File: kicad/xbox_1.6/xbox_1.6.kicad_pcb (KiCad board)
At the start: 2 copper layers, 18 parts, among them U2C1 intel_495_bga2, U4B1 ddr_100_tqfp, U4C1 nvidia_xgpu_nv2a, U5F1 ddr_100_tqfp, U6D1 ddr_100_tqfp, U6E1 nvidia_mcpx

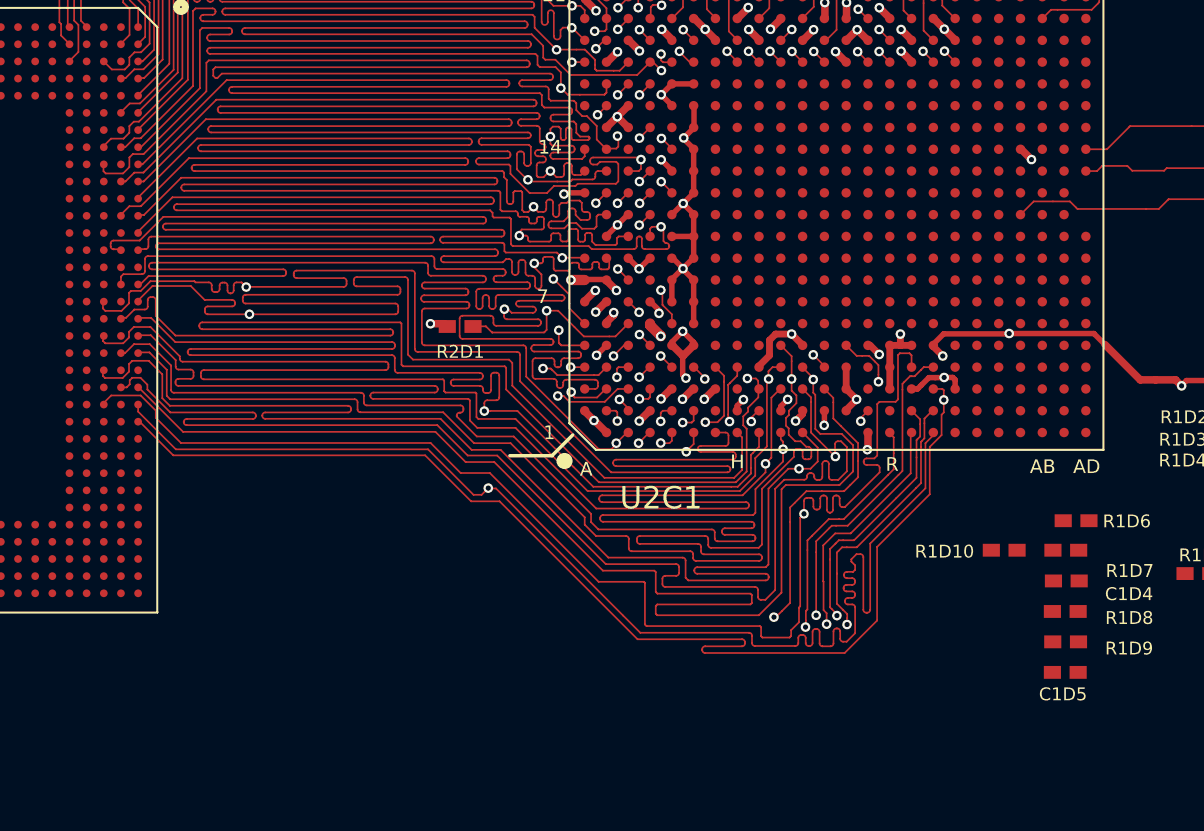
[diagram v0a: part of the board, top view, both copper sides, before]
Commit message: route more
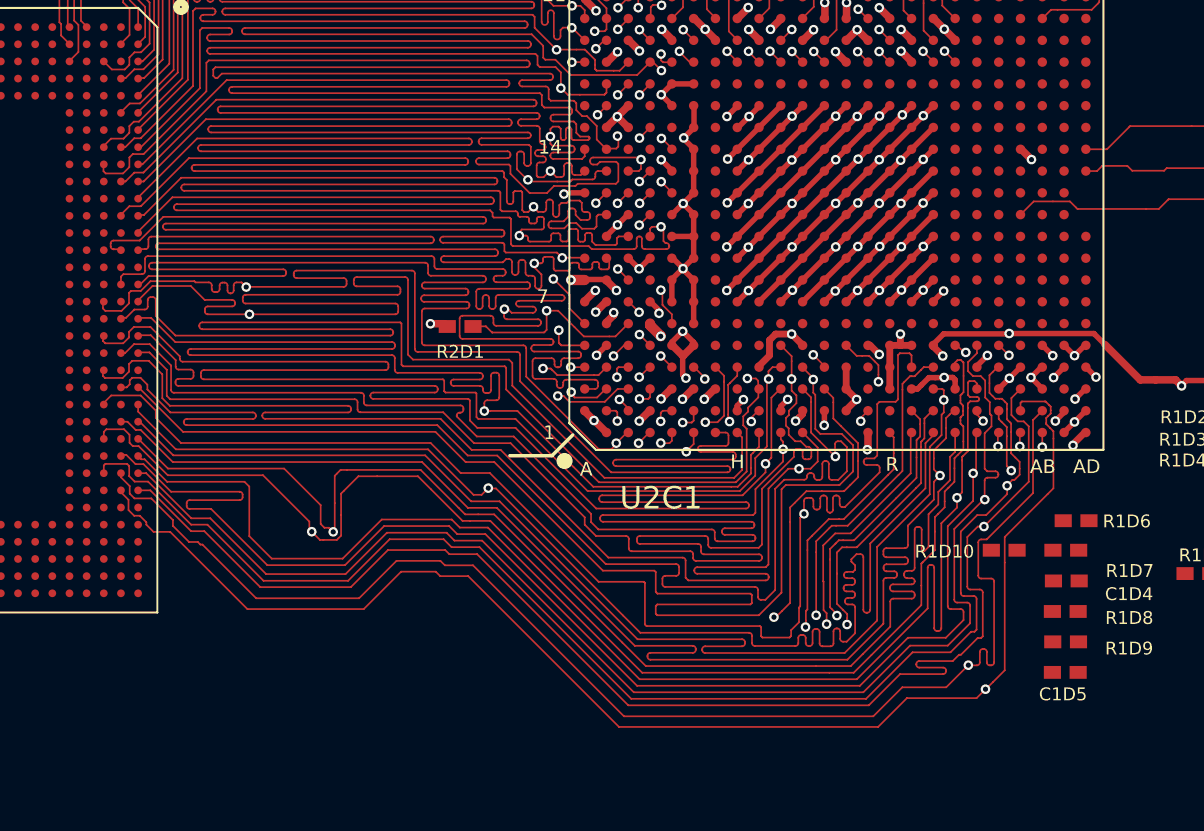
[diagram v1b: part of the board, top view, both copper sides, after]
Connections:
- U2C1 pad AA1: (no net) -> /CPU_AERR
- U2C1 pad AA2: (no net) -> /CPU_RS1
- U2C1 pad AA3: (no net) -> /CPU_DBSY
- U2C1 pad AA4: (no net) -> /VSS
- U2C1 pad AB1: (no net) -> /CPU_AP0
- U2C1 pad AB2: (no net) -> /CPU_ADS
- U2C1 pad AB3: (no net) -> /VSS
- U2C1 pad AB4: (no net) -> /VSS
- U2C1 pad AB5: (no net) -> /VSS
- U2C1 pad AC1: (no net) -> /VSS
- U2C1 pad AC2: (no net) -> /VSS
- U2C1 pad AC4: (no net) -> /VSS
- U2C1 pad AC5: (no net) -> /VSS
- U2C1 pad AD1: (no net) -> /VSS
- U2C1 pad AD2: (no net) -> /VSS
- U2C1 pad AD3: (no net) -> /VSS
- U2C1 pad AD4: (no net) -> /VSS
- U2C1 pad AD5: (no net) -> /VSS
- U2C1 pad H10: (no net) -> /CPU_VCC
- U2C1 pad H11: (no net) -> /VSS
- U2C1 pad H12: (no net) -> /CPU_VCC
- U2C1 pad H13: (no net) -> /VSS
- U2C1 pad H14: (no net) -> /CPU_VCC
- U2C1 pad H15: (no net) -> /VSS
- U2C1 pad H16: (no net) -> /CPU_VCC
- U2C1 pad H7: (no net) -> /VSS
- U2C1 pad H8: (no net) -> /CPU_VCC
- U2C1 pad H9: (no net) -> /VSS
- U2C1 pad J10: (no net) -> /VSS
- U2C1 pad J11: (no net) -> /CPU_VCC
- U2C1 pad J12: (no net) -> /VSS
- U2C1 pad J13: (no net) -> /CPU_VCC
- U2C1 pad J14: (no net) -> /VSS
- U2C1 pad J15: (no net) -> /CPU_VCC
- U2C1 pad J16: (no net) -> /VSS
- U2C1 pad J6: (no net) -> /CPU_VCCT
- U2C1 pad J7: (no net) -> /CPU_VCC
- U2C1 pad J8: (no net) -> /VSS
- U2C1 pad J9: (no net) -> /CPU_VCC
- U2C1 pad K10: (no net) -> /CPU_VCC
- U2C1 pad K11: (no net) -> /VSS
- U2C1 pad K12: (no net) -> /CPU_VCC
- U2C1 pad K13: (no net) -> /VSS
- U2C1 pad K14: (no net) -> /CPU_VCC
- U2C1 pad K15: (no net) -> /VSS
- U2C1 pad K16: (no net) -> /CPU_VCC
- U2C1 pad K7: (no net) -> /VSS
- U2C1 pad K8: (no net) -> /CPU_VCC
- U2C1 pad K9: (no net) -> /VSS
- U2C1 pad L10: (no net) -> /VSS
- U2C1 pad L11: (no net) -> /CPU_VCC
- U2C1 pad L12: (no net) -> /VSS
- U2C1 pad L13: (no net) -> /CPU_VCC
- U2C1 pad L14: (no net) -> /VSS
- U2C1 pad L15: (no net) -> /CPU_VCC
- U2C1 pad L16: (no net) -> /VSS
- U2C1 pad L7: (no net) -> /CPU_VCC
- U2C1 pad L8: (no net) -> /VSS
- U2C1 pad L9: (no net) -> /CPU_VCC
- U2C1 pad M10: (no net) -> /CPU_VCC
- U2C1 pad M11: (no net) -> /VSS
- U2C1 pad M12: (no net) -> /CPU_VCC
- U2C1 pad M13: (no net) -> /VSS
- U2C1 pad M14: (no net) -> /CPU_VCC
- U2C1 pad M15: (no net) -> /VSS
- U2C1 pad M16: (no net) -> /CPU_VCC
- U2C1 pad M7: (no net) -> /VSS
- U2C1 pad M8: (no net) -> /CPU_VCC
- U2C1 pad M9: (no net) -> /VSS
- U2C1 pad N10: (no net) -> /VSS
- U2C1 pad N11: (no net) -> /CPU_VCC
- U2C1 pad N12: (no net) -> /VSS
- U2C1 pad N13: (no net) -> /CPU_VCC
- U2C1 pad N14: (no net) -> /VSS
- U2C1 pad N15: (no net) -> /CPU_VCC
- U2C1 pad N16: (no net) -> /VSS
- U2C1 pad N7: (no net) -> /CPU_VCC
- U2C1 pad N8: (no net) -> /VSS
- U2C1 pad N9: (no net) -> /CPU_VCC
- U2C1 pad P10: (no net) -> /CPU_VCC
- U2C1 pad P11: (no net) -> /VSS
- U2C1 pad P12: (no net) -> /CPU_VCC
- U2C1 pad P13: (no net) -> /VSS
- U2C1 pad P14: (no net) -> /CPU_VCC
- U2C1 pad P15: (no net) -> /VSS
- U2C1 pad P16: (no net) -> /CPU_VCC
- U2C1 pad P7: (no net) -> /VSS
- U2C1 pad P8: (no net) -> /CPU_VCC
- U2C1 pad P9: (no net) -> /VSS
- U2C1 pad R10: (no net) -> /VSS
- U2C1 pad R11: (no net) -> /CPU_VCC
- U2C1 pad R12: (no net) -> /VSS
- U2C1 pad R13: (no net) -> /CPU_VCC
- U2C1 pad R14: (no net) -> /VSS
- U2C1 pad R15: (no net) -> /CPU_VCC
- U2C1 pad R16: (no net) -> /VSS
- U2C1 pad R7: (no net) -> /CPU_VCC
- U2C1 pad R8: (no net) -> /VSS
- U2C1 pad R9: (no net) -> /CPU_VCC
- U2C1 pad T10: (no net) -> /CPU_VCC
- U2C1 pad T11: (no net) -> /VSS
- U2C1 pad T12: (no net) -> /CPU_VCC
- U2C1 pad T13: (no net) -> /VSS
- U2C1 pad T14: (no net) -> /CPU_VCC
- U2C1 pad T15: (no net) -> /VSS
- U2C1 pad T16: (no net) -> /CPU_VCC
- U2C1 pad T7: (no net) -> /VSS
- U2C1 pad T8: (no net) -> /CPU_VCC
- U2C1 pad T9: (no net) -> /VSS
- U2C1 pad U10: (no net) -> /VSS
- U2C1 pad U11: (no net) -> /CPU_VCC
- U2C1 pad U12: (no net) -> /VSS
- U2C1 pad U13: (no net) -> /CPU_VCC
- U2C1 pad U14: (no net) -> /VSS
- U2C1 pad U15: (no net) -> /CPU_VCC
- U2C1 pad U16: (no net) -> /VSS
- U2C1 pad U7: (no net) -> /CPU_VCC
- U2C1 pad U8: (no net) -> /VSS
- U2C1 pad U9: (no net) -> /CPU_VCC
- U2C1 pad V1: (no net) -> /CPU_HIT
- U2C1 pad V2: (no net) -> /CPU_REQ2
- U2C1 pad V4: (no net) -> /CPU_REQ1
- U2C1 pad V5: (no net) -> /CPU_PWRGOOD
- U2C1 pad W1: (no net) -> /CPU_RS2
- U2C1 pad W2: (no net) -> /CPU_RP
- U2C1 pad W3: (no net) -> /CPU_REQ3
- U2C1 pad W4: (no net) -> /VSS
- U2C1 pad W5: (no net) -> /CPU_REQ4
- U2C1 pad Y1: (no net) -> /CPU_RSP
- U2C1 pad Y2: (no net) -> /CPU_AP1
- U2C1 pad Y3: (no net) -> /VSS
- U2C1 pad Y4: (no net) -> /CPU_HITM
- U2C1 pad Y5: (no net) -> /CPU_TESTLO1
- U4C1 pad A25: (no net) -> /CPU_HIT
- U4C1 pad A26: (no net) -> /CPU_REQ3
- U4C1 pad A27: (no net) -> /CPU_REQ4
- U4C1 pad A28: (no net) -> /CPU_DBSY
- U4C1 pad B24: (no net) -> /CPU_REQ2
- U4C1 pad B26: (no net) -> /CPU_RS2
- U4C1 pad B27: (no net) -> /CPU_ADS
- U4C1 pad B28: (no net) -> /CPU_RS1
- U4C1 pad C25: (no net) -> /CPU_REQ1
- U4C1 pad C27: (no net) -> /CPU_HITM
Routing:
- net /VSS: track 79.5 -> 166.6 mm, vias 47 -> 83
- net /CPU_REQ3: track 0.00 -> 80.7 mm, vias 0 -> 1
- net /CPU_HITM: track 0.00 -> 80.1 mm, vias 0 -> 1
- net /CPU_RS1: track 0.00 -> 80.1 mm, vias 0 -> 1
- net /CPU_ADS: track 0.00 -> 79.3 mm, vias 0 -> 1
- net /CPU_DBSY: track 0.00 -> 79.2 mm, vias 0 -> 1
- net /CPU_REQ4: track 0.00 -> 77.7 mm, vias 0 -> 1
- net /CPU_RS2: track 0.00 -> 77.4 mm, vias 0 -> 1
- net /CPU_REQ1: track 0.00 -> 77.0 mm, vias 0 -> 1
- net /CPU_VCC: track 0.00 -> 76.9 mm, vias 0 -> 16
- net /CPU_REQ2: track 0.00 -> 75.8 mm, vias 0 -> 1
- net /CPU_HIT: track 0.00 -> 75.7 mm, vias 0 -> 1
- net /CPU_AP1: track 0.00 -> 3.79 mm, vias 0 -> 1
- net /CPU_AP0: track 0.00 -> 0.85 mm, vias 0 -> 1
- net /CPU_TESTLO1: track 0.00 -> 0.84 mm, vias 0 -> 1
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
